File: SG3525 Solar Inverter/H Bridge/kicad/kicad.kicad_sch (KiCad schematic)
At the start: 78 parts, among them J2 Screw_Terminal_01x02, J3 Screw_Terminal_01x02, J4 Screw_Terminal_01x02, Q1 IRF740, Q2 IRF740, Q3 S8050, Q4 S8050, Q5 IRF740, Q6 IRF740, U1 SG3525, U2 PC817, U3 LM358, U4 PC817

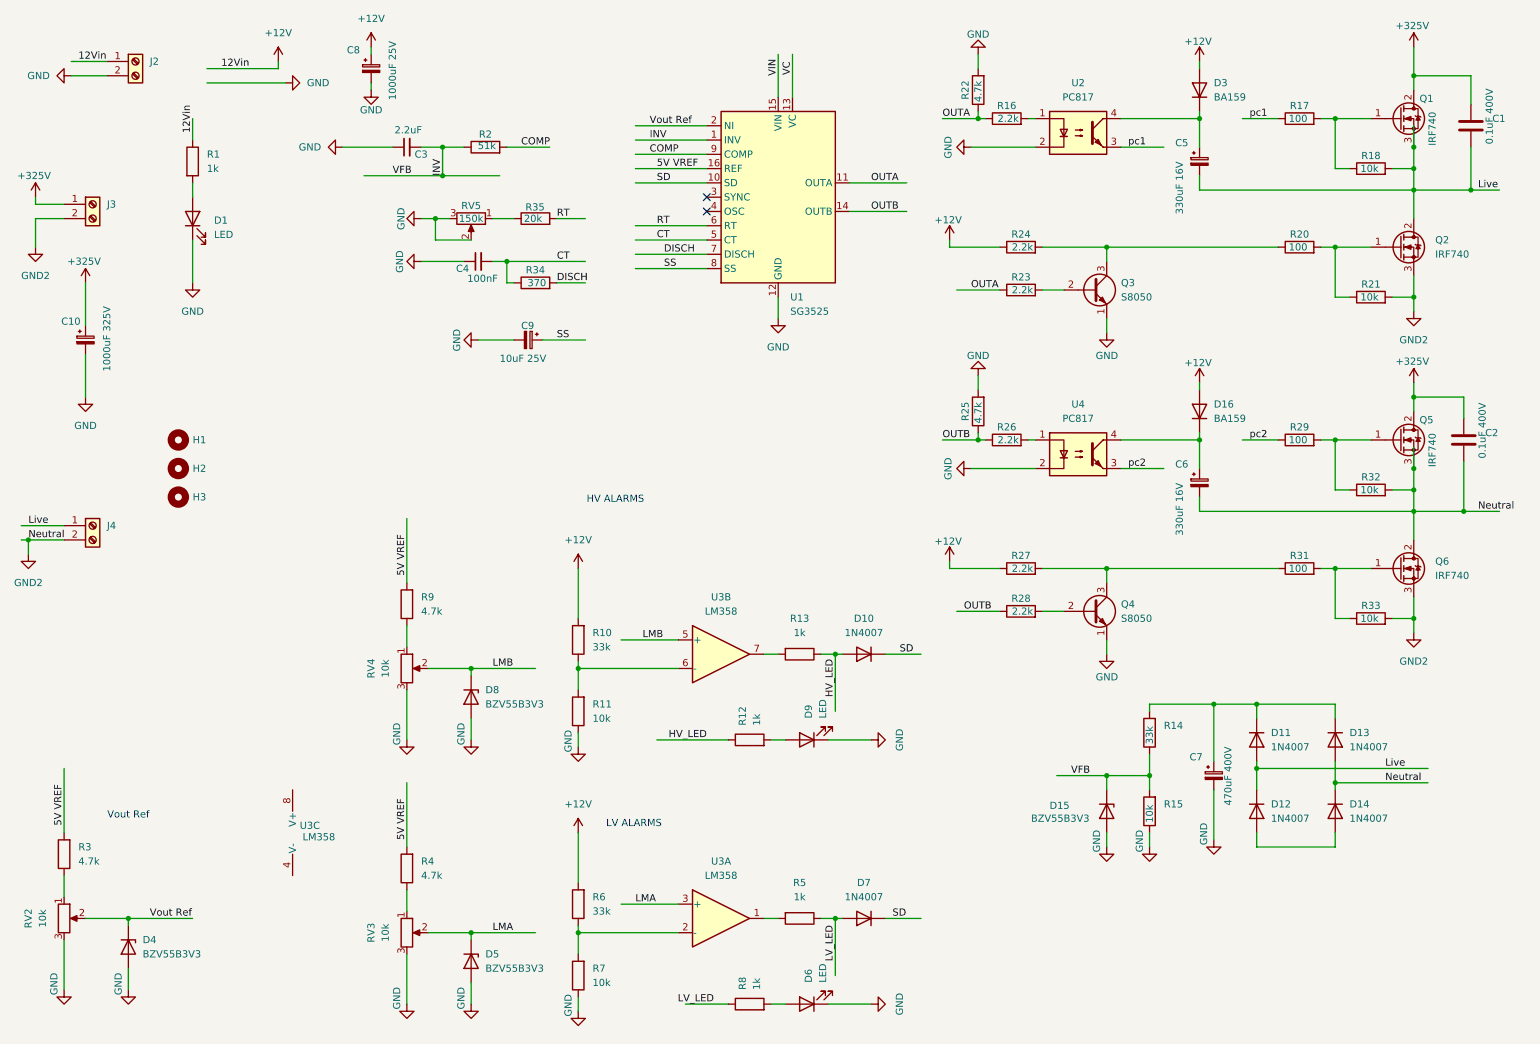
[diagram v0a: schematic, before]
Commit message: WORKING ON H Bridge kicad
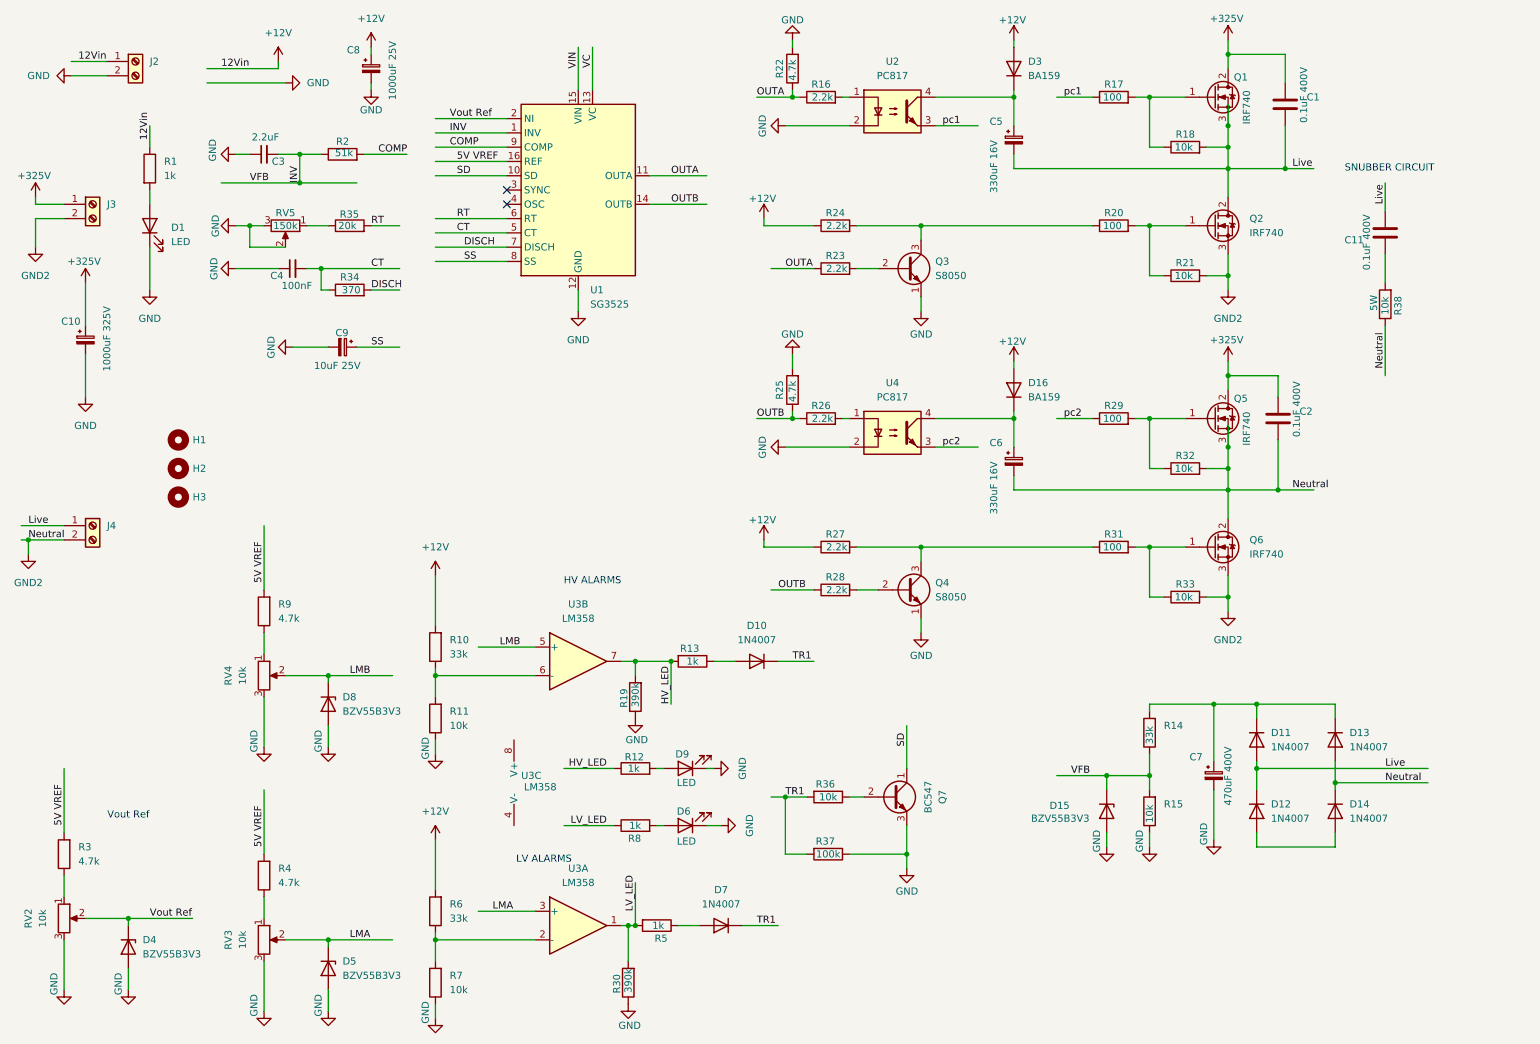
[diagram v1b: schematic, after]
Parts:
- added C11: 0.1uF 400V, Capacitor_THT:C_Rect_L13.5mm_W5.0mm_P10.00mm_FKS3_FKP3_MKS4, symbol Device:C
- added Q7: BC547, Package_TO_SOT_THT:TO-92_Inline, symbol Transistor_BJT:BC547
- added R19, R30: 390k, Resistor_THT:R_Axial_DIN0207_L6.3mm_D2.5mm_P7.62mm_Horizontal, symbol Device:R
- added R36, R38: 10k, Resistor_THT:R_Axial_DIN0207_L6.3mm_D2.5mm_P7.62mm_Horizontal, symbol Device:R
- added R37: 100k, Resistor_THT:R_Axial_DIN0207_L6.3mm_D2.5mm_P7.62mm_Horizontal, symbol Device:R
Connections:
- net GND: now also Q7.3 (E), R19.1, R30.1, R37.1
- net GND2: now also R38.1
- net HV_LED: now also R13.2, U3.7, R19.2; no longer D10.2 (A), R13.1
- net LV_LED: now also R5.2, U3.1, R30.2; no longer D7.2 (A), R5.1
- net Live: now also C11.2
- net SD: now also Q7.1 (C); no longer D10.1 (K), D7.1 (K)
- new net: D10.2 (A), R13.1
- new net: Q7.2 (B), R36.1
- new net: D7.2 (A), R5.1
- new net: C11.1, R38.2
- new net TR1: D10.1 (K), D7.1 (K), R36.2, R37.2
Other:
- note added: "SNUBBER CIRCUIT"
- moved on the sheet: C1, C2, C3, C4, C5, C6, C9, D1, D10, D16, D3, D5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
